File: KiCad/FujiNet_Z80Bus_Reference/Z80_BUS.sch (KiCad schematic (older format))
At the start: 10 parts, among them IC21 7432N, IC22 7432N, J1 HOST SYSTEM HEADER

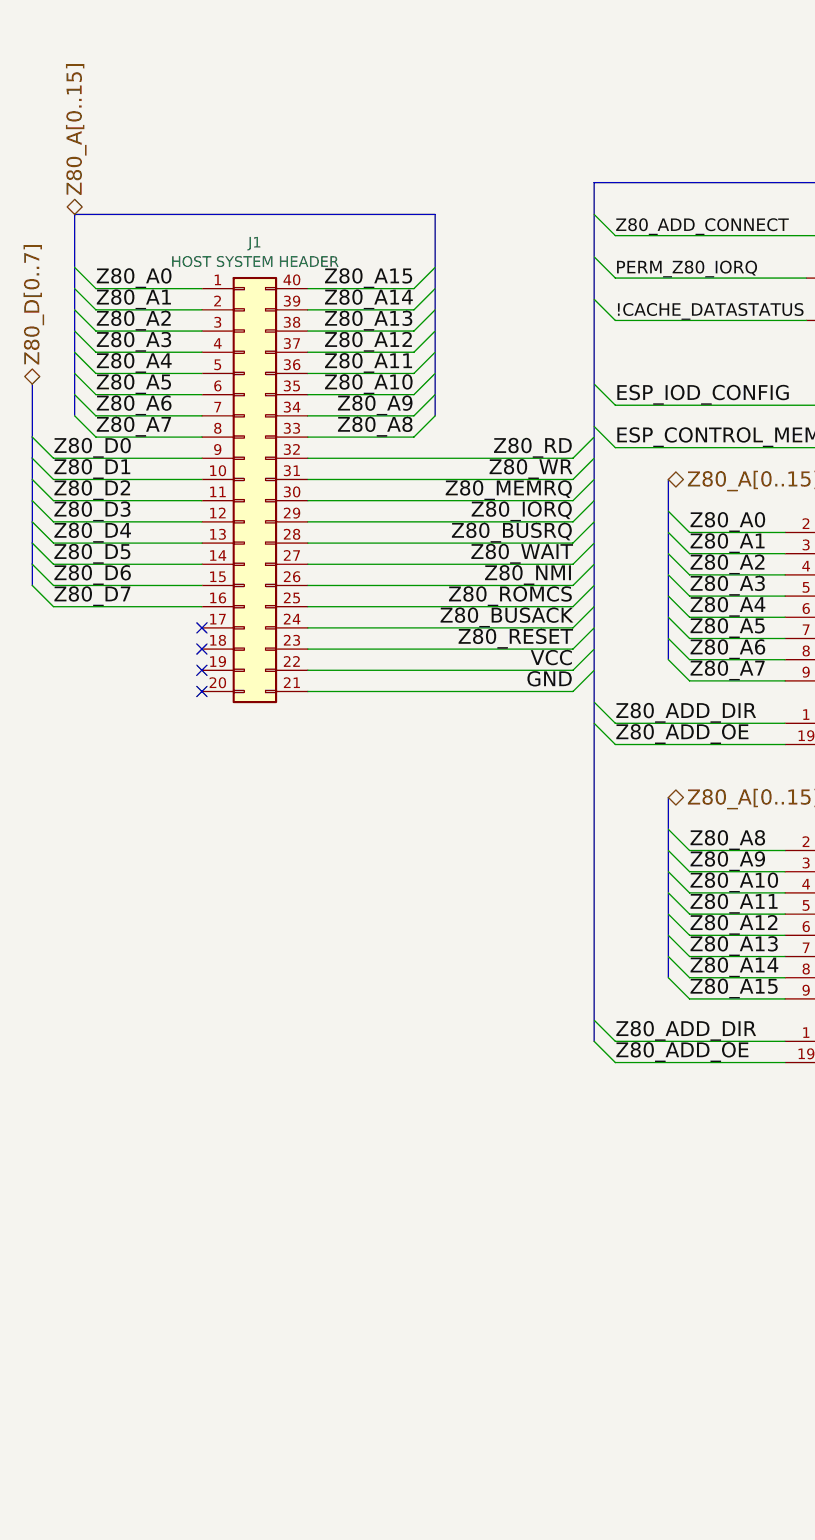
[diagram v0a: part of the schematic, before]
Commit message: Last KiCad5 commit
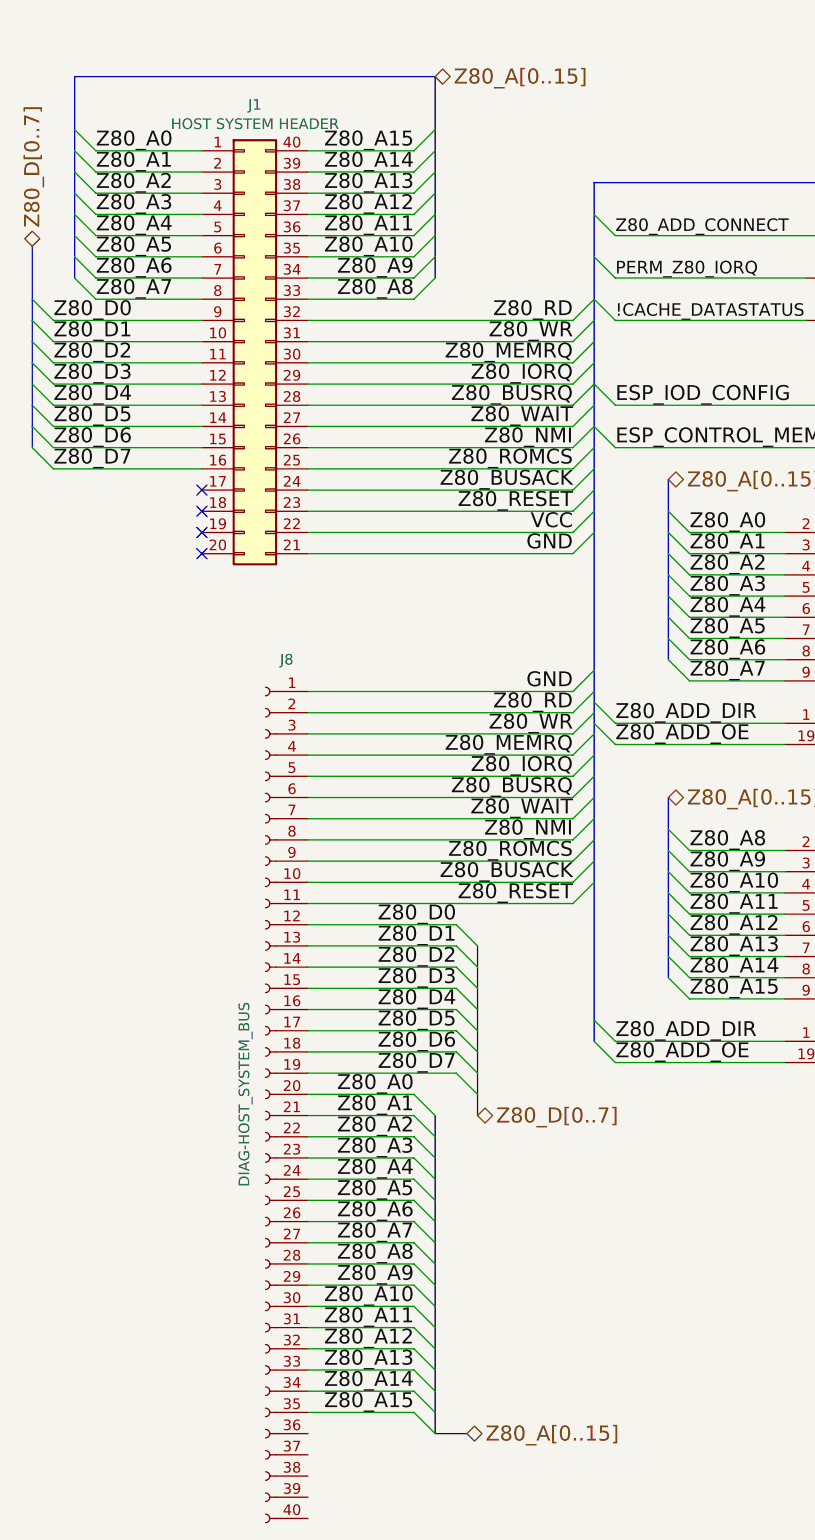
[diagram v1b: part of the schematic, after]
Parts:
- added J8: DIAG-HOST_SYSTEM_BUS, Connector_PinHeader_2.54mm:PinHeader_1x40_P2.54mm_Vertical, symbol Connector:Conn_01x40_Female
- J1: footprint Connector_PinHeader_2.54mm:PinHeader_1x40_P2.54mm_Vertical -> Connector_PinHeader_2.54mm:PinHeader_2x20_P2.54mm_Vertical
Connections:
- net GND: now also J8.1 (Pin_1)
- net Z80_A0: now also J8.20 (Pin_20)
- net Z80_A1: now also J8.21 (Pin_21)
- net Z80_A10: now also J8.30 (Pin_30)
- net Z80_A11: now also J8.31 (Pin_31)
- net Z80_A12: now also J8.32 (Pin_32)
- net Z80_A13: now also J8.33 (Pin_33)
- net Z80_A14: now also J8.34 (Pin_34)
- net Z80_A15: now also J8.35 (Pin_35)
- net Z80_A2: now also J8.22 (Pin_22)
- net Z80_A3: now also J8.23 (Pin_23)
- net Z80_A4: now also J8.24 (Pin_24)
- net Z80_A5: now also J8.25 (Pin_25)
- net Z80_A6: now also J8.26 (Pin_26)
- net Z80_A7: now also J8.27 (Pin_27)
- net Z80_A8: now also J8.28 (Pin_28)
- net Z80_A9: now also J8.29 (Pin_29)
- net Z80_BUSACK: now also J8.10 (Pin_10)
- net Z80_BUSRQ: now also J8.6 (Pin_6)
- net Z80_D0: now also J8.12 (Pin_12)
- net Z80_D1: now also J8.13 (Pin_13)
- net Z80_D2: now also J8.14 (Pin_14)
- net Z80_D3: now also J8.15 (Pin_15)
- net Z80_D4: now also J8.16 (Pin_16)
- net Z80_D5: now also J8.17 (Pin_17)
- net Z80_D6: now also J8.18 (Pin_18)
- net Z80_D7: now also J8.19 (Pin_19)
- net Z80_IORQ: now also J8.5 (Pin_5)
- net Z80_MEMRQ: now also J8.4 (Pin_4)
- net Z80_NMI: now also J8.8 (Pin_8)
- net Z80_RD: now also J8.2 (Pin_2)
- net Z80_RESET: now also J8.11 (Pin_11)
- net Z80_ROMCS: now also J8.9 (Pin_9)
- net Z80_WAIT: now also J8.7 (Pin_7)
- net Z80_WR: now also J8.3 (Pin_3)
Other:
- moved on the sheet: J1
